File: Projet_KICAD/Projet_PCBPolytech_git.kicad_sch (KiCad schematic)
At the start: 14 parts, among them J1 Conn_01x05_Socket, J2 USB_B_Micro, SW1 SW_Push, U1 STM32F446RETx, U2 USBLC6-2SC6

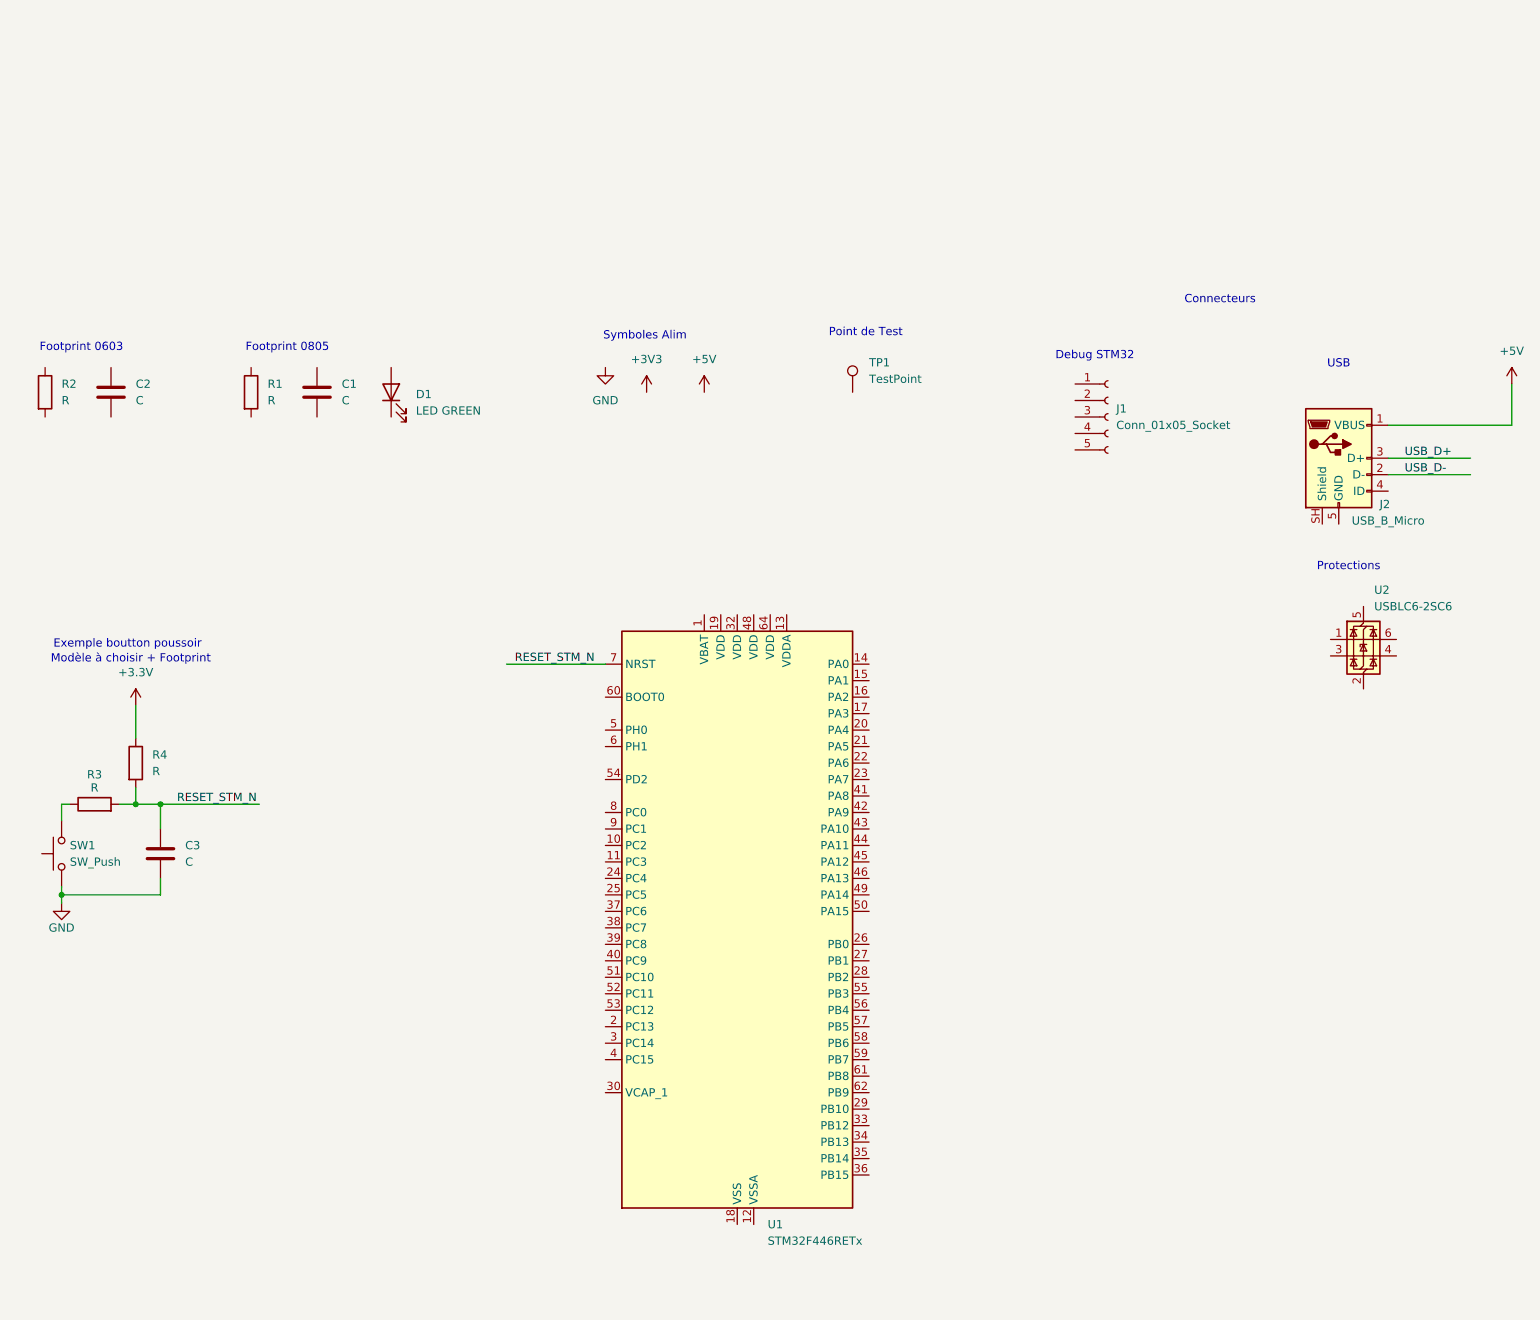
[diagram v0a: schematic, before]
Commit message: Update Projet_PCBPolytech_git.kicad_sch
Mise à jour du schéma STM32F405 et alimentation
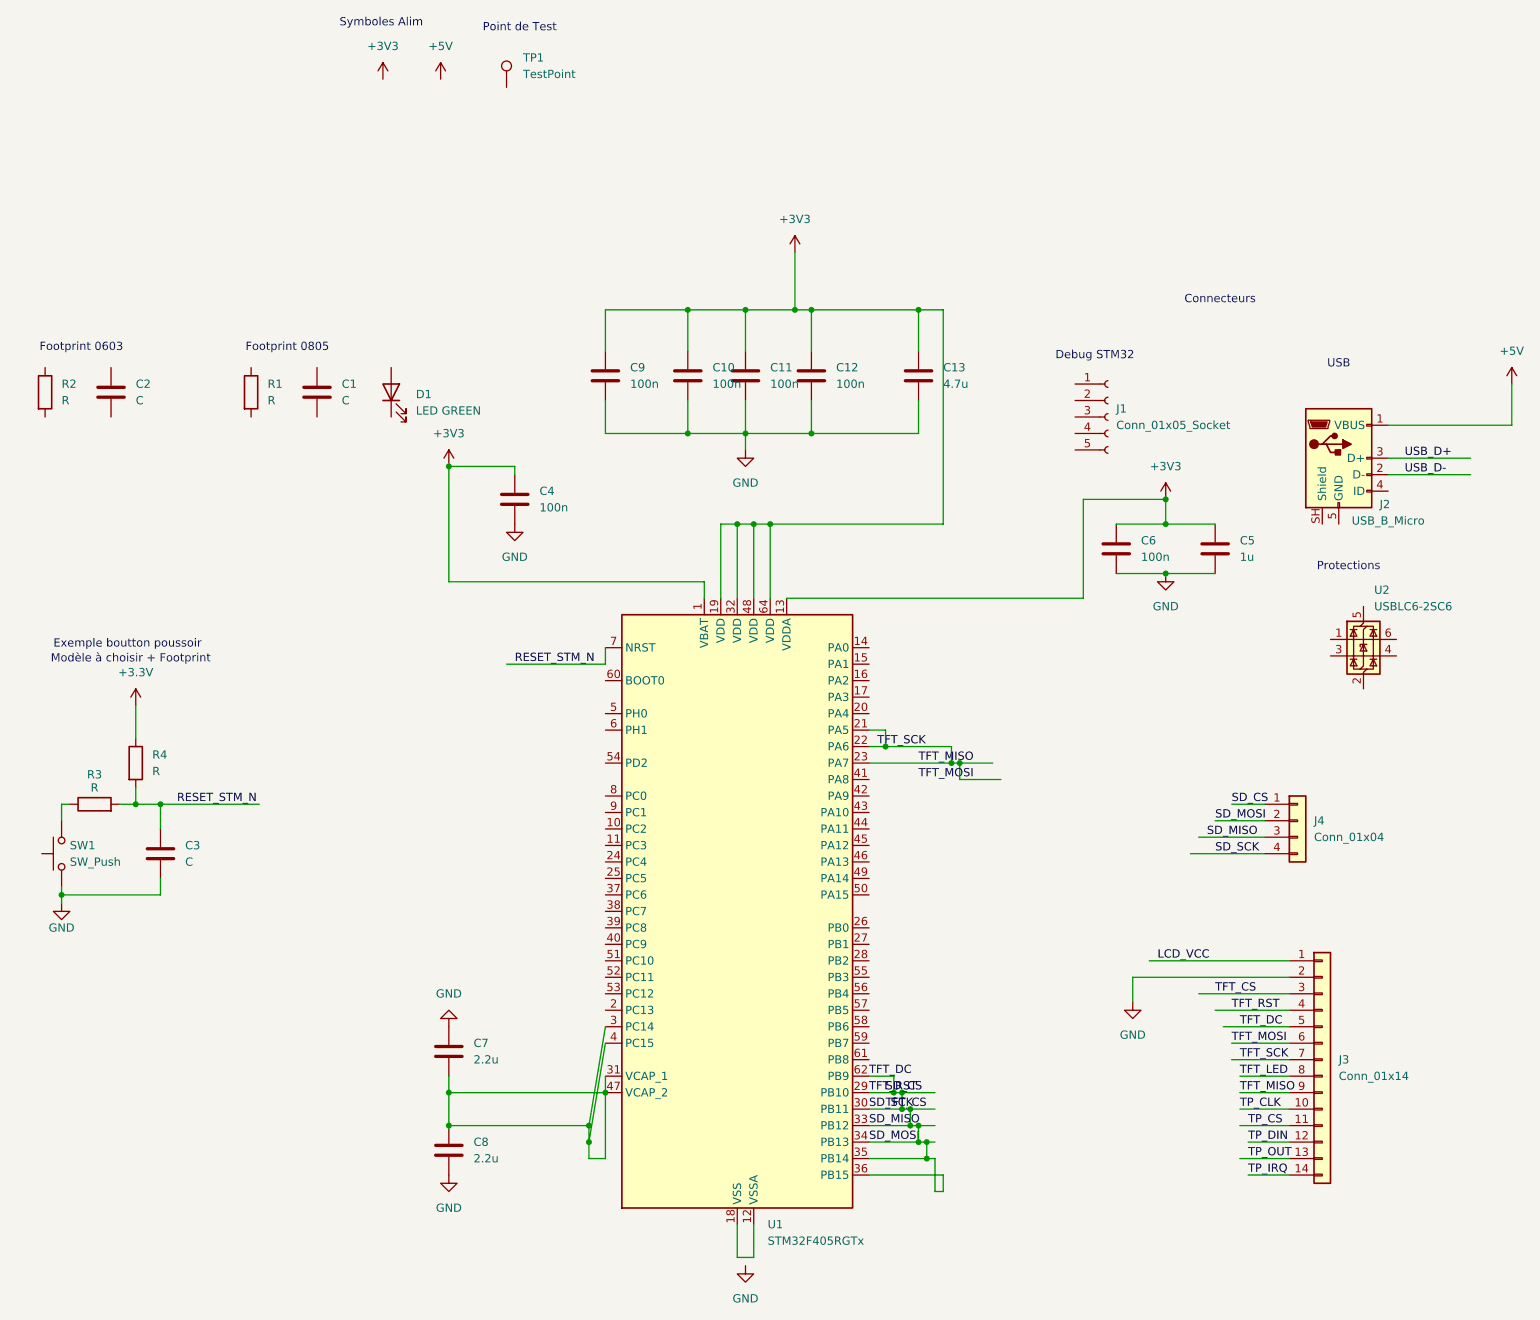
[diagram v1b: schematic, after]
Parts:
- added C10, C11, C12, C9: 100n, Capacitor_SMD:C_0805_2012Metric, symbol Device:C
- added C13: 4.7u, Capacitor_SMD:C_0805_2012Metric, symbol Device:C
- added C4, C6: 100n, C_0805_2012Metric, symbol Device:C
- added C5: 1u, Capacitor_SMD:C_0805_2012Metric, symbol Device:C
- added C7, C8: 2.2u, Capacitor_SMD:C_0805_2012Metric, symbol Device:C
- added J3: Conn_01x14, symbol Connector_Generic:Conn_01x14
- added J4: Conn_01x04, symbol Connector_Generic:Conn_01x04
- U1: value STM32F446RETx -> STM32F405RGTx; symbol MCU_ST_STM32F4:STM32F446RETx -> MCU_ST_STM32F4:STM32F405RGTx; LCSC Part # (none) -> C15742
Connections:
- net +3V3: now also U1.1 (VBAT), U1.13 (VDDA), U1.19 (VDD), U1.32 (VDD), U1.48 (VDD), U1.64 (VDD), C10.1, C11.1, C12.1, C13.1, C4.1, C5.1, C6.1, C9.1
- net GND: now also C10.2, C11.2, C12.2, C13.2, C4.2, C5.2, C6.2, C7.1, C8.2, C9.2, J3.2 (Pin_2)
- net at U1.12 (VSSA): now also U1.18 (VSS), U1.63 (VSS)
- net at U1.31 (VCAP_1), U1.47 (VCAP_2): now also U1.3 (PC14), U1.4 (PC15), C7.2, C8.1; no longer U1.18 (VSS), U1.63 (VSS)
- net TFT_MISO: now reaches U1.21 (PA5)
- net TFT_MISO: now also U1.22 (PA6), U1.23 (PA7), J3.7 (Pin_7), J3.9 (Pin_9)
- net SD_CS: now reaches U1.29 (PB10)
- net SD_CS: now also U1.30 (PB11), U1.33 (PB12), U1.34 (PB13), U1.35 (PB14), U1.36 (PB15), U1.62 (PB9), J3.3 (Pin_3), J3.4 (Pin_4), J3.5 (Pin_5), J4.1 (Pin_1), J4.2 (Pin_2), J4.3 (Pin_3), J4.4 (Pin_4)
- new net LCD_VCC: J3.1 (Pin_1)
- new net TFT_LED: J3.8 (Pin_8)
- new net TFT_MOSI: J3.6 (Pin_6)
- new net TP_CLK: J3.10 (Pin_10)
- new net TP_CS: J3.11 (Pin_11)
- new net TP_DIN: J3.12 (Pin_12)
- new net TP_IRQ: J3.14 (Pin_14)
- new net TP_OUT: J3.13 (Pin_13)
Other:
- moved on the sheet: TP1
